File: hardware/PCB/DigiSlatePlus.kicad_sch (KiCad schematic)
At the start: 40 parts, among them J1 Serial, J10 IO7, J2 USB_B, J6 Mains, J7 Timecode IN, J8 Timecode OUT, J9 MISO, Q4 2N2222, SW1 RotaryEncoder-SW, SW2 1, SW3 1, SW4 1, SW5 1, SW6 BOOT, U1 ESP32-S3-WROOM-1, U2 DS3231M

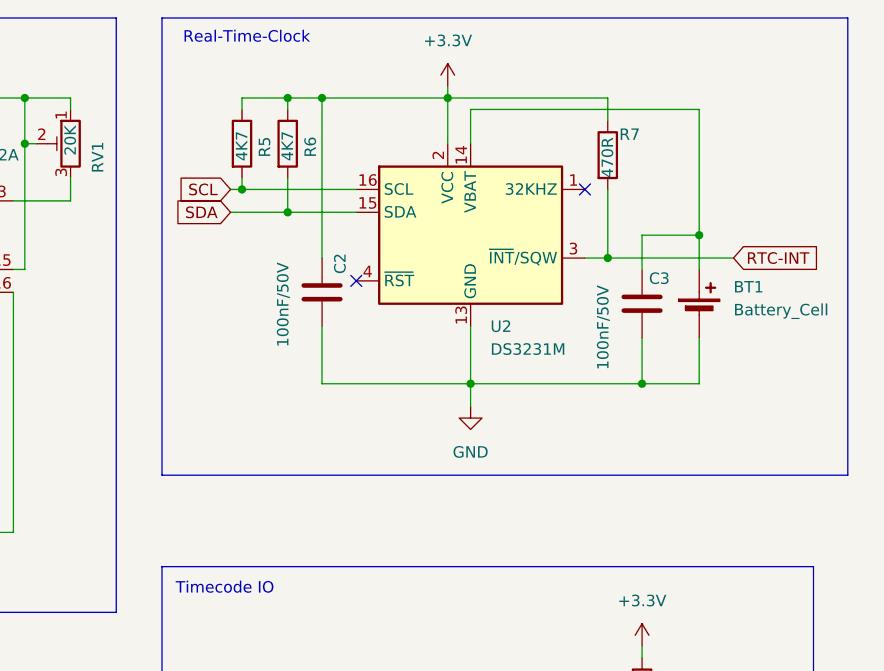
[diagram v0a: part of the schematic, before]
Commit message: bugfixes in board
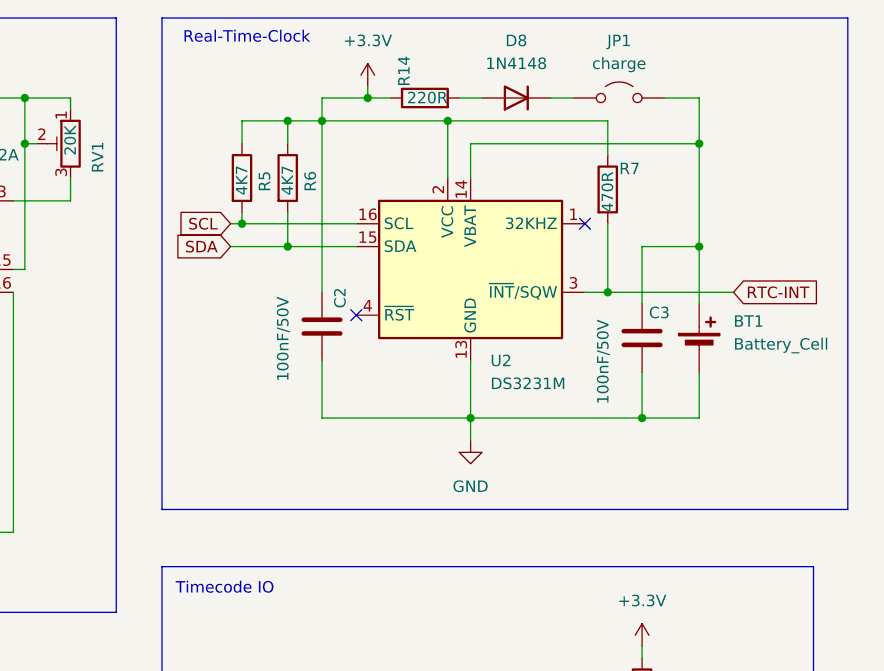
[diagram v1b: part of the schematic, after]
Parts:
- added D8: 1N4148, Diode_SMD:D_PowerDI-123, symbol Diode:1N4148
- added JP1: charge, Jumper:SolderJumper-2_P1.3mm_Open_TrianglePad1.0x1.5mm, symbol Jumper:Jumper_2_Open
- added R14: 220R, Resistor_SMD:R_1206_3216Metric, symbol Device:R
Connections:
- net +3.3V: now also R14.1
- net at BT1.1 (+), C3.1, U2.14 (VBAT): now also JP1.2 (B)
- new net: D8.1 (K), JP1.1 (A)
- new net: D8.2 (A), R14.2
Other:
- moved on the sheet: BT1, C2, C3, R5, R6, R7, U2
